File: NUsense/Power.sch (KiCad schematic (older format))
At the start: 36 parts, among them Q1201 BC807, Q1202 2N3055, Q1203 Q_NMOS_GDS, Q1204 Q_NMOS_GDS, Q1205 2N2219, Q1206 Q_PMOS_GDS, SW1201 SW_SPDT, U1201 LD1086D2M33

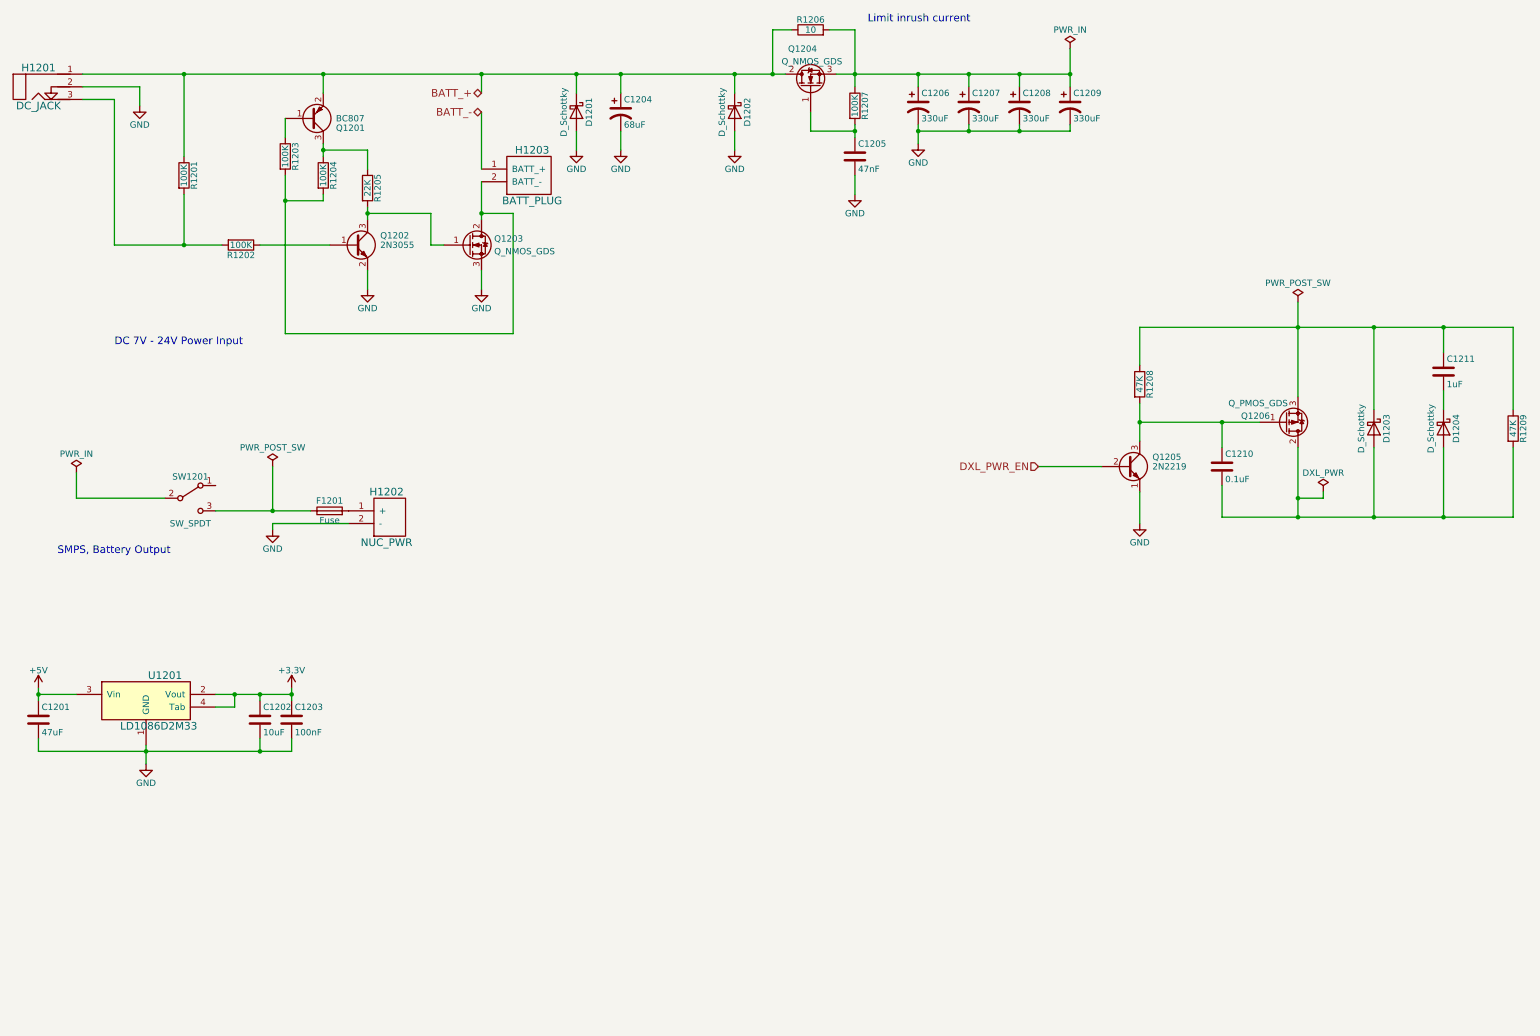
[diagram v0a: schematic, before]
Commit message: Cleans up some minor things
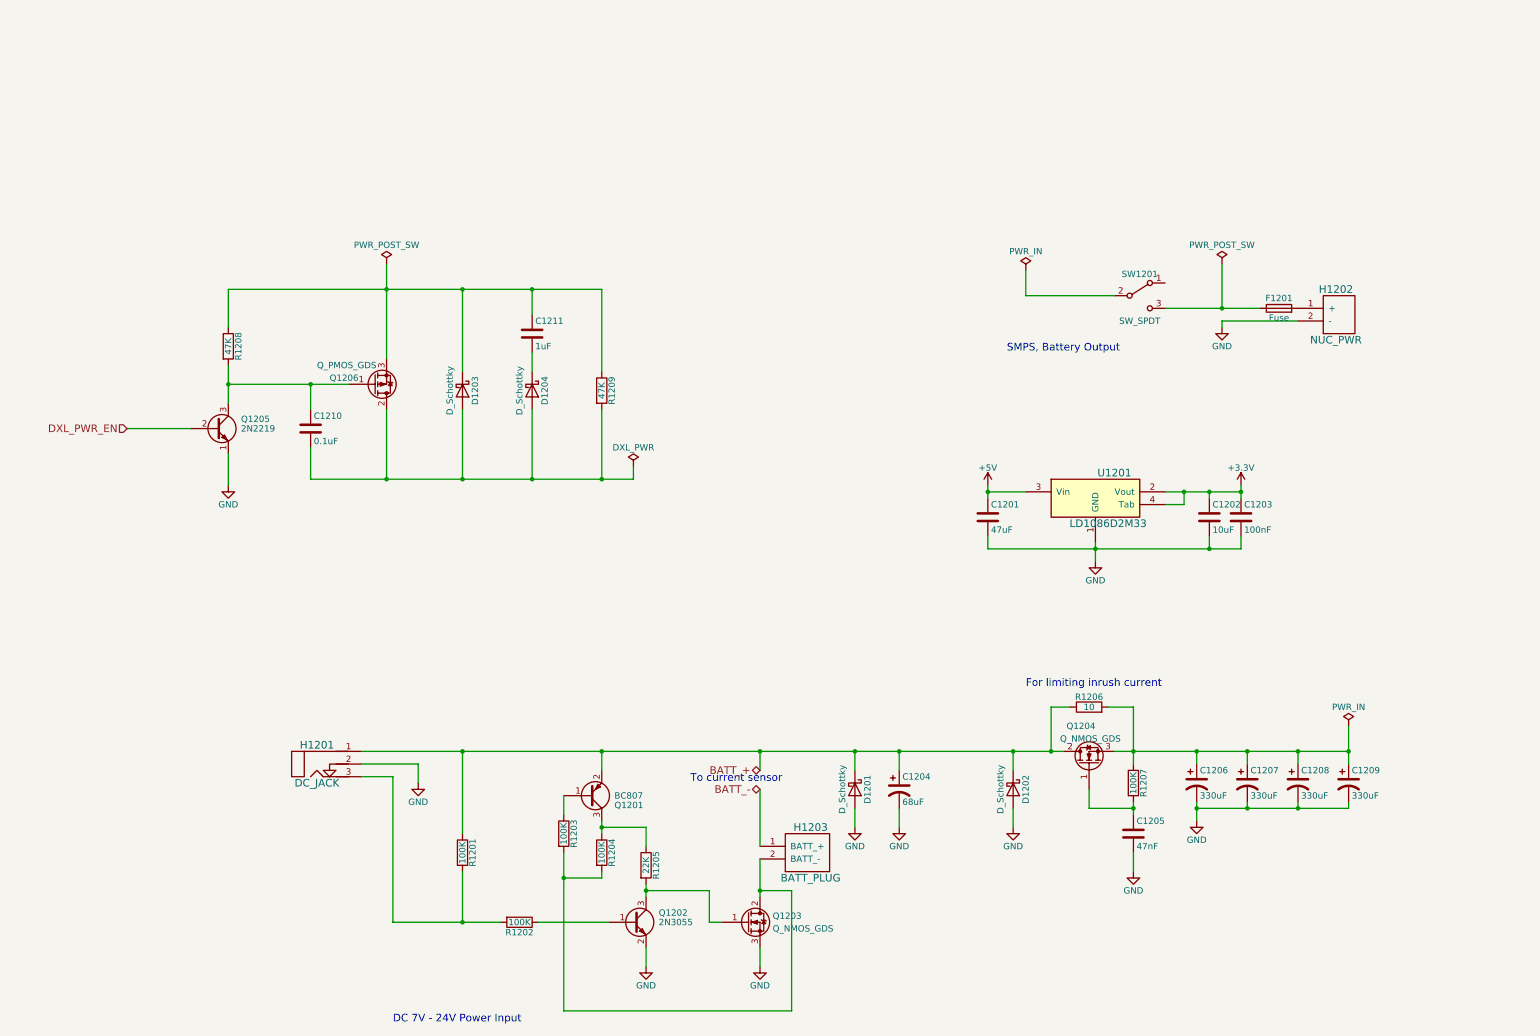
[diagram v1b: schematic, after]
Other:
- note added: "For limiting inrush current"
- note added: "To current sensor"
- note removed: "Limit inrush current"
- moved on the sheet: C1201, C1202, C1203, C1204, C1205, C1206, C1207, C1208, C1209, C1210, C1211, D1201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
